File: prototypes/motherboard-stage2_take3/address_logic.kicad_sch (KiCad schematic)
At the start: 13 parts, among them U23 GAL 22V10, U24 74LS670, U25 74LS670, U26 GAL 22V10, U27 GAL16V8, U28 74HC245

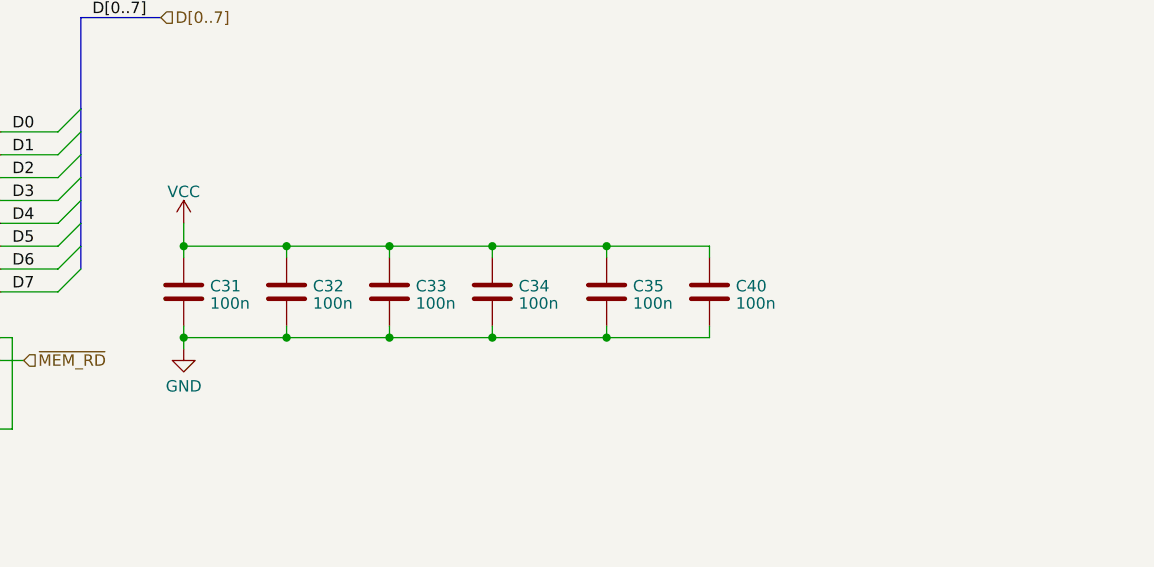
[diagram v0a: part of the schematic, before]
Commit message: Finalized stage 2
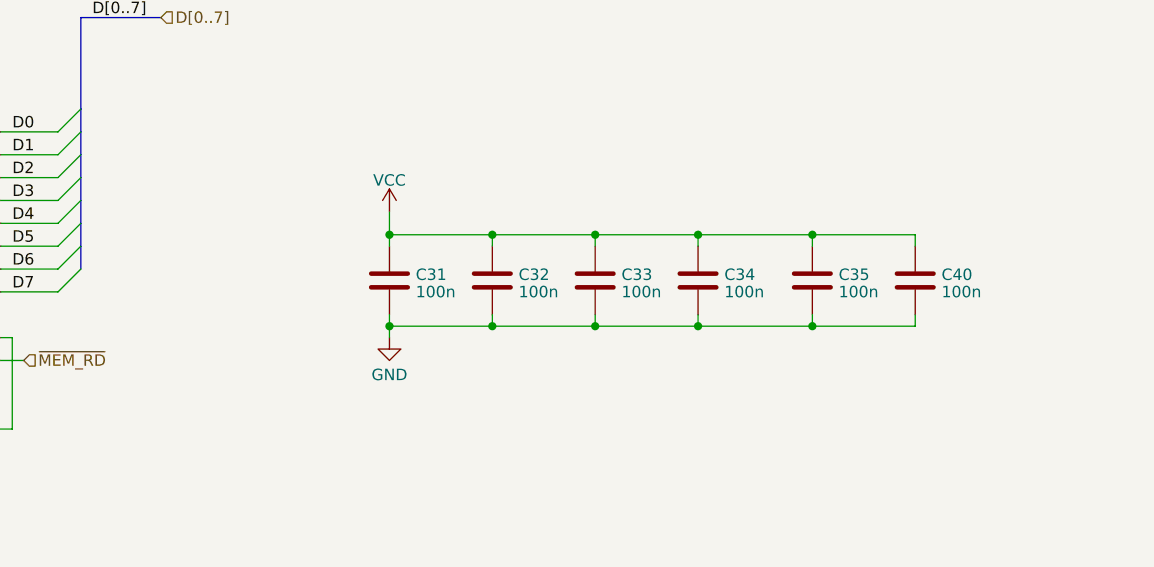
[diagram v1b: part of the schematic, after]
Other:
- moved on the sheet: C31, C32, C33, C34, C35, C40
